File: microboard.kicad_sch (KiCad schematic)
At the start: 81 parts, among them J1 Conn_02x01, J10 Conn_02x01, J11 Conn_02x01, J12 Conn_01x10, J13 Conn_02x01, J14 Conn_01x03, J15 Conn_02x01, J16 Conn_02x01, J17 Conn_02x01, J18 Conn_02x01, J19 Conn_02x01, J2 Conn_01x10, J20 Conn_02x01, J21 Conn_01x01_Socket, J22 Conn_01x01_Socket, J3 Conn_01x10, J39 Conn_01x10, J4 USB_C_Receptacle_USB2.0, J40 Conn_01x10, J41 Conn_01x10, J42 Conn_02x01, J43 Conn_01x05, J44 Conn_01x09, J45 Conn_01x08, J5 Conn_01x04, J6 Conn_01x02, J7 Conn_01x03, J8 Conn_01x10, J9 Conn_02x01, SW1 SW_Push, SW2 SW_Push, SW3 SW_Push, SW4 SW_Push, U1 USBLC6-2SC6, U2 ATSAMD21G18A-AUT, U4 TXS0108EPW, U5 LD1117S12TR_SOT223, U6 LD1117S50TR_SOT223, Y1 32768Hz

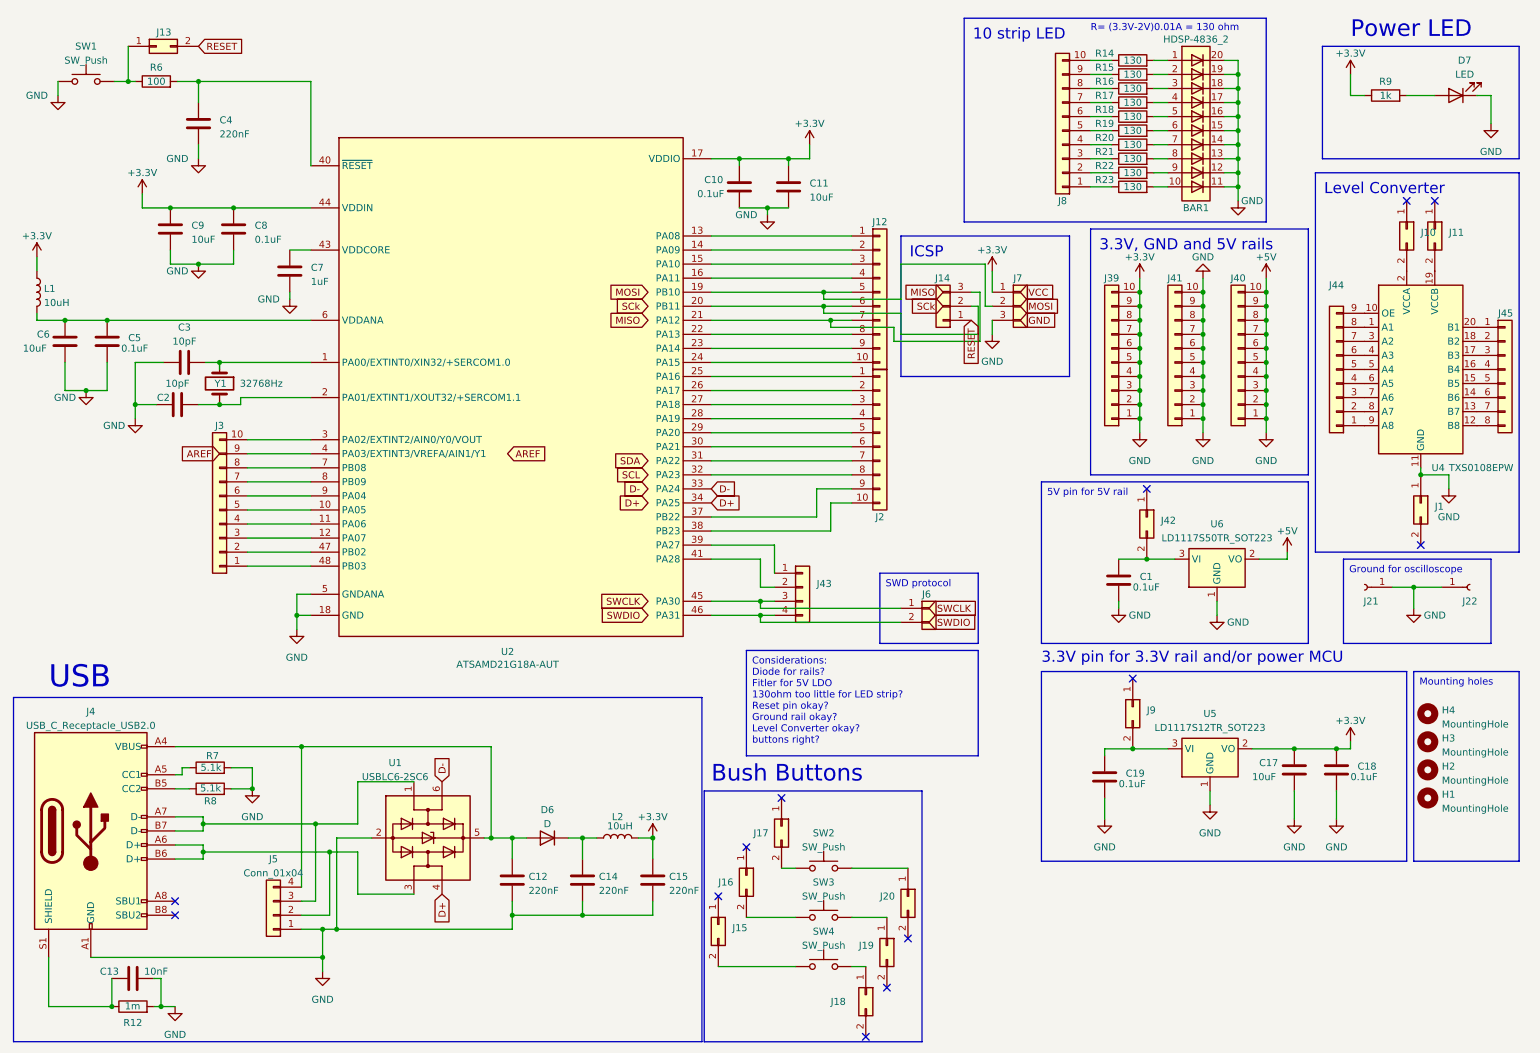
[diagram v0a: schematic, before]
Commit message: Add files via upload
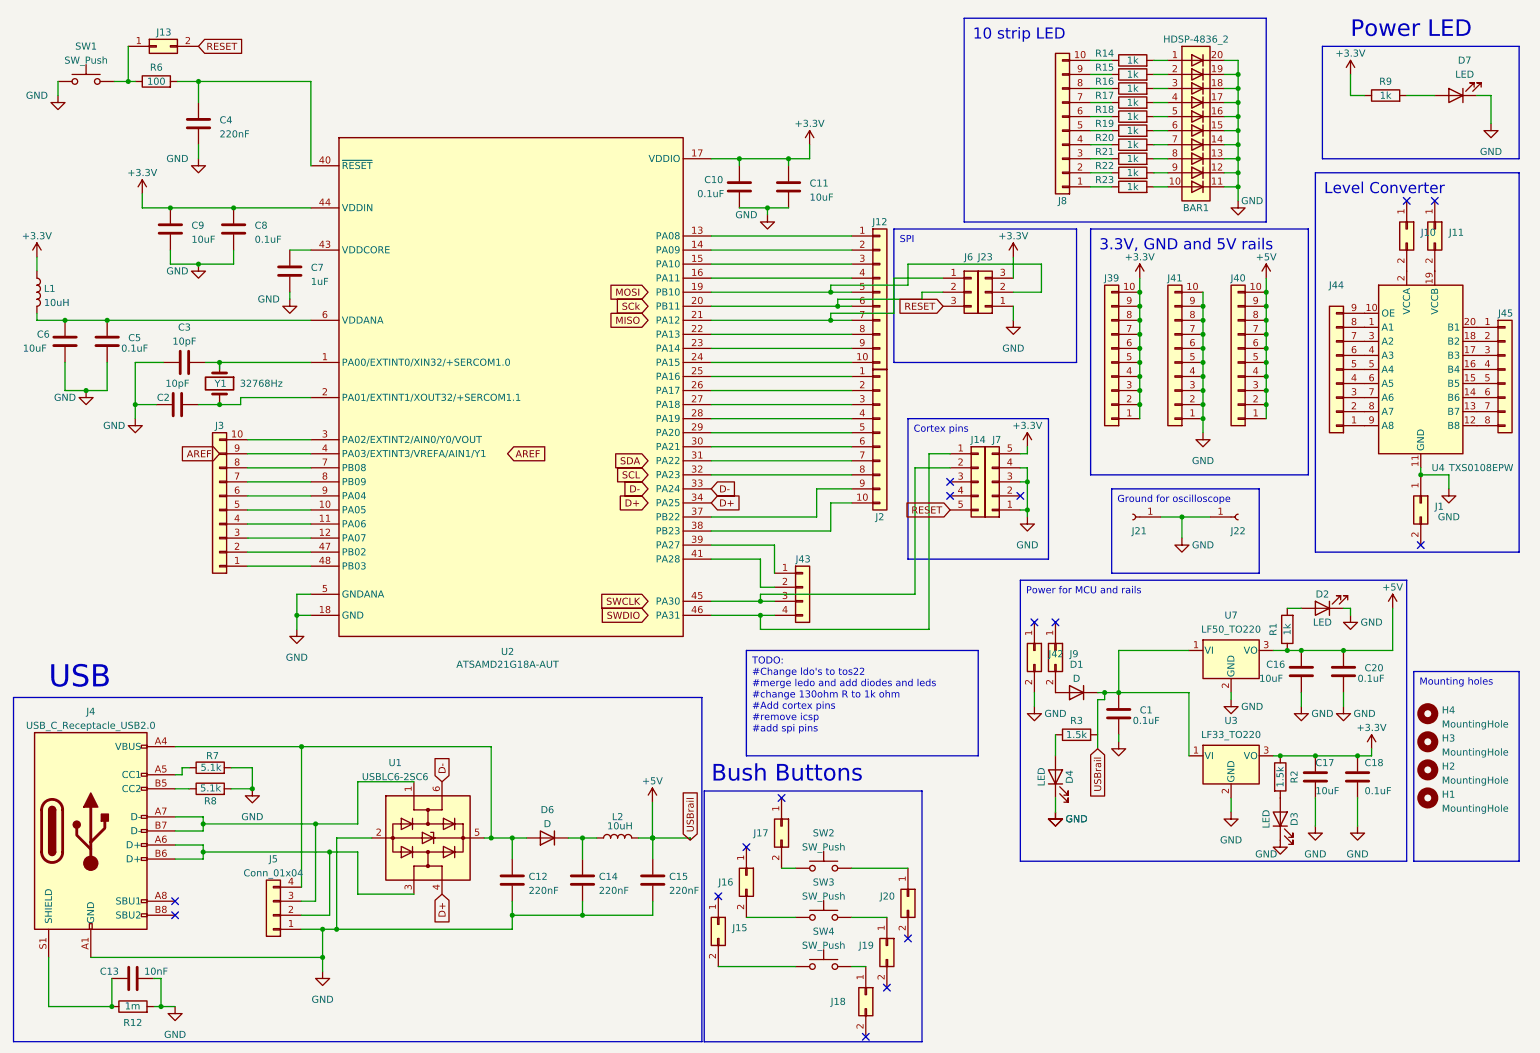
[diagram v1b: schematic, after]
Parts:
- removed C19: 0.1uF, symbol Device:C
- removed J14, J7: Conn_01x03, symbol Connector_Generic:Conn_01x03
- removed J6: Conn_01x02, symbol Connector_Generic:Conn_01x02
- removed U5: LD1117S12TR_SOT223, Package_TO_SOT_SMD:SOT-223-3_TabPin2, symbol Regulator_Linear:LD1117S12TR_SOT223
- removed U6: LD1117S50TR_SOT223, Package_TO_SOT_SMD:SOT-223-3_TabPin2, symbol Regulator_Linear:LD1117S50TR_SOT223
- added C16: 10uF, symbol Device:C
- added C20: 0.1uF, symbol Device:C
- added D1: D, symbol Device:D
- added D2, D3, D4: LED, symbol Device:LED
- added J14, J7: Conn_01x05, symbol Connector_Generic:Conn_01x05
- added J23, J6: Conn_01x03, symbol Connector_Generic:Conn_01x03
- added R1: 1k, symbol Device:R
- added R2, R3: 1.5k, symbol Device:R
- added U3: LF33_TO220, Package_TO_SOT_THT:TO-220-3_Vertical, symbol Regulator_Linear:LF33_TO220
- added U7: LF50_TO220, Package_TO_SOT_THT:TO-220-3_Vertical, symbol Regulator_Linear:LF50_TO220
- R14, R15, R16, R17, R18, R19, R20, R21, R22, R23: value 130 -> 1k
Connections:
- net +3.3V: now also J14.5 (Pin_5), J23.3 (Pin_3), R2.1, U3.3 (VO); no longer BAR1.11 (K), BAR1.12 (K), BAR1.13 (K), BAR1.14 (K), BAR1.15 (K), BAR1.16 (K), BAR1.17 (K), BAR1.18 (K), BAR1.19 (K), BAR1.20 (K), C1.2, C10.2, C11.2, C12.2, C13.2, C14.2, C15.1, C15.2, C17.2, C18.2, C2.1, C3.2, C4.2, C5.2, C6.2, C7.2, C8.2, C9.2, D7.1 (K), J1.1 (Pin_1), J21.1 (Pin_1), J22.1 (Pin_1), J4.A1 (GND), J4.A12 (GND), J4.B1 (GND), J4.B12 (GND), J40.1 (Pin_1), J40.10 (Pin_10), J40.2 (Pin_2), J40.3 (Pin_3), J40.4 (Pin_4), J40.5 (Pin_5), J40.6 (Pin_6), J40.7 (Pin_7), J40.8 (Pin_8), J40.9 (Pin_9), J41.1 (Pin_1), J41.10 (Pin_10), J41.2 (Pin_2), J41.3 (Pin_3), J41.4 (Pin_4), J41.5 (Pin_5), J41.6 (Pin_6), J41.7 (Pin_7), J41.8 (Pin_8), J41.9 (Pin_9), J5.1 (Pin_1), L2.2, R12.2, R7.2, R8.2, SW1.1, U1.2 (GND), U2.18 (GND), U2.35 (GND), U2.42 (GND), U2.5 (GNDANA), U4.11 (GND)
- net RESET: now also J6.3 (Pin_3), J7.5 (Pin_5)
- net at J9.2 (Pin_2): now also D1.2 (A)
- net at J43.3 (Pin_3), U2.45 (PA30): now also J7.2 (Pin_2)
- net at J43.4 (Pin_4), U2.46 (PA31): now also J7.1 (Pin_1)
- net at J12.5 (Pin_5), U2.19 (PB10): now also J23.2 (Pin_2)
- net at J12.6 (Pin_6), U2.20 (PB11): now also J6.2 (Pin_2)
- net at J12.7 (Pin_7), U2.21 (PA12): now also J6.1 (Pin_1)
- net +5V: now reaches C1.1
- net +5V: now also C15.1, J40.1 (Pin_1), J40.10 (Pin_10), J40.2 (Pin_2), J40.3 (Pin_3), J40.4 (Pin_4), J40.5 (Pin_5), J40.6 (Pin_6), J40.7 (Pin_7), J40.8 (Pin_8), J40.9 (Pin_9), L2.2, C16.1, C20.1, D1.1 (K), R1.1, U3.1 (VI), U7.1 (VI), U7.3 (VO); no longer J42.2 (Pin_2)
- new net: D3.2 (A), R2.2
- new net: D4.2 (A), R3.1
- new net: D2.2 (A), R1.2
- new net GND: BAR1.11 (K), BAR1.12 (K), BAR1.13 (K), BAR1.14 (K), BAR1.15 (K), BAR1.16 (K), BAR1.17 (K), BAR1.18 (K), BAR1.19 (K), BAR1.20 (K), C1.2, C10.2, C11.2, C12.2, C13.2, C14.2, C15.2, C16.2, C17.2, C18.2, C2.1, C20.2, C3.2, C4.2, C5.2, C6.2, C7.2, C8.2, C9.2, D2.1 (K), D3.1 (K), D4.1 (K), D7.1 (K), J1.1 (Pin_1), J14.1 (Pin_1), J14.3 (Pin_3), J14.4 (Pin_4), J21.1 (Pin_1), J22.1 (Pin_1), J23.1 (Pin_1), J4.A1 (GND), J4.A12 (GND), J4.B1 (GND), J4.B12 (GND), J41.1 (Pin_1), J41.10 (Pin_10), J41.2 (Pin_2), J41.3 (Pin_3), J41.4 (Pin_4), J41.5 (Pin_5), J41.6 (Pin_6), J41.7 (Pin_7), J41.8 (Pin_8), J41.9 (Pin_9), J42.2 (Pin_2), J5.1 (Pin_1), R12.2, R7.2, R8.2, SW1.1, U1.2 (GND), U2.18 (GND), U2.35 (GND), U2.42 (GND), U2.5 (GNDANA), U3.2 (GND), U4.11 (GND), U7.2 (GND)
- no-connect marks 13 -> 16
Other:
- note removed: "3.3V pin for 3.3V rail and/or power MCU"
- note removed: "R= (3.3V-2V)0.01A = 130 ohm"
- title: JeffUino -> Dev_MCU_Board
- moved on the sheet: C17, C18, J21, J22, J42, J9
